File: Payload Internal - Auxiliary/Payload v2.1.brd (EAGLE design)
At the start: 90.5 x 91.8 mm, 11 parts, among them J30 M80-866XXXX, J31 M80-866XXXX

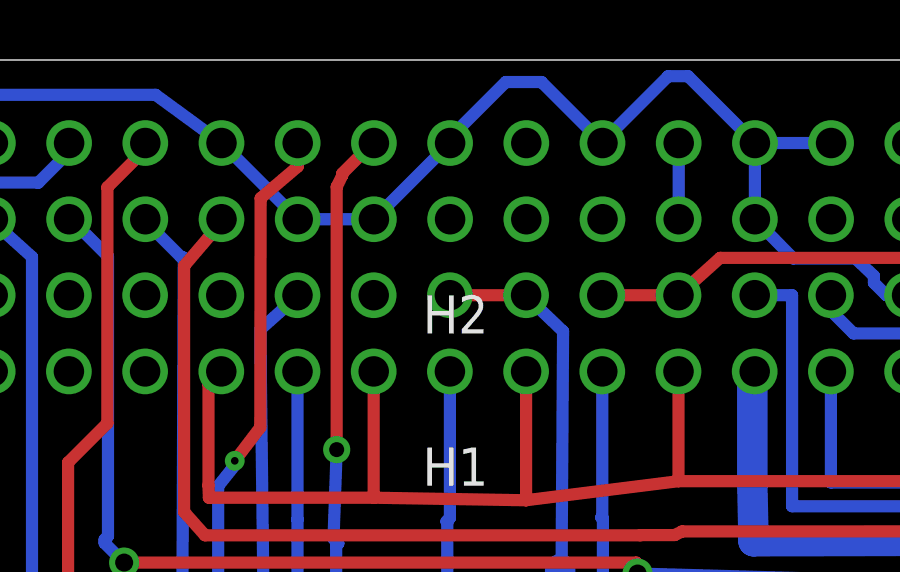
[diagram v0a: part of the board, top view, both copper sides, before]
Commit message: Revert "Fixed all the trivial wiring issues for the CDH, Diplexer, EPS and wiring harness schematics"
This reverts commits
  6713d85a6277b26f983fd7a52d0f95a7f9e4e046.
  086194ae58682b6763f31692a26cd4dac33df983
  82b42737f0fe6cd82dfea4a4ae7507beb01cc7b8

This revert is required because changing/connecting net names in eagle will automatically modify or destroy PCB traces associated with those netnames.
Updating the schematics and PCBs will need to be redone carefully to ensure no traces are destroyed.

	modified:   CDH-V3.7/CDH-v3.7.brd
	modified:   CDH-V3.7/CDH-v3.7.sch
	modified:   Diplexer/diplexer_v4rev0-schematic.sch
	modified:   EPS/eps-v1-0.brd
	modified:   EPS/eps-v1-0.sch
	modified:   Payload Internal - Auxiliary/Payload v2.1.brd
	modified:   Payload Internal - Auxiliary/Payload v2.1.sch
	modified:   Wiring Harness/wiring-harness-complete-v1.0.sch
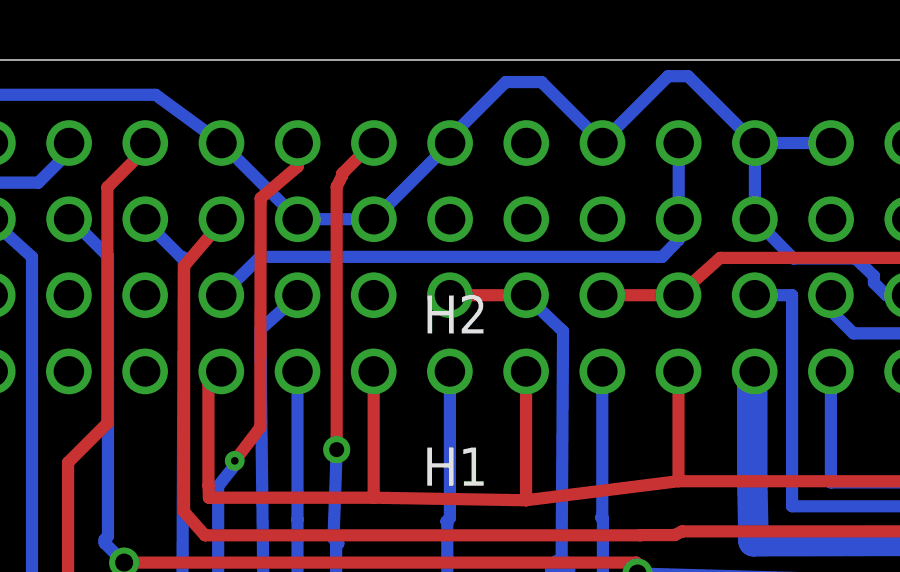
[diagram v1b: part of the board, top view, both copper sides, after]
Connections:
- net BATTERY_THRMSTOR1_+V renamed BATTERY_THRMSTOR_+V
- net BATTERY_THRMSTOR2_+V renamed BATTERY_THERMSTOR_2+
- net POW_9V renamed 9V
- net POW_RADIO_VBATT renamed POW_5V
- net THERMALGND1 renamed THERMALGND
- removed net EXTERNAL_POWER_V+: H2.52
- removed net N$1: H2.6
- removed net N$6: H2.10
- removed net POW_RADIO_3V3: H2.27, H2.28
- new net EXTERNAL_POWER_+V: H2.51
- new net N$19: H2.37
- new net N$89.: H2.21
- new net N$90: H2.23
- new net N$91: H2.25
- net EXTERNAL_POWER_GND: now also H2.52; no longer H2.51
- net N$4: now also H2.35; no longer H2.8
- net POW_RADIO_3.3V: now also H2.27, H2.28
- net Q6_SPI_SCLK: now also H2.6; no longer H2.21
- net Q6_SPI_SDI_MISO: now also H2.10; no longer H2.35
- net Q6_SPI_SDO_MOSI: now also H2.8; no longer H2.23
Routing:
- net POW_RADIO_3.3V: track 0.00 -> 19.2 mm
- net POW_RADIO_3V3: track 2.54 -> 0.00 mm
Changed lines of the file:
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@@
 <?xml version="1.0" encoding="utf-8"?>
 <!DOCTYPE eagle SYSTEM "eagle.dtd">
-<eagle version="7.3.0">
+<eagle version="7.2.0">
 <drawing>
 <settings>
@@
 <contactref element="H2" pad="47"/>
 </signal>
+<signal name="N$19">
+<contactref element="H2" pad="37"/>
+</signal>
 <signal name="N$22">
 <contactref element="H2" pad="34"/>
+</signal>
+<signal name="N$90">
+<contactref element="H2" pad="23"/>
 </signal>
 <signal name="N$27">
@@
 <contactref element="H1" pad="33"/>
 </signal>
+<signal name="Q6_SPI_SDO_MOSI">
+<contactref element="H2" pad="8"/>
+</signal>
 <signal name="Q6_SPI_CS1">
 <contactref element="H2" pad="12"/>
@@
 </polygon>
 </signal>
-<signal name="POW_RADIO_VBATT">
+<signal name="POW_5V">
 <contactref element="H1" pad="28"/>
 <contactref element="H1" pad="26"/>
@@
 <wire x1="81.331828125" y1="77.2444875" x2="82.066653125" y2="76.5096625" width="0.4064" layer="1"/>
 </signal>
+<signal name="N$89.">
+<contactref element="H2" pad="21"/>
+</signal>
+<signal name="Q6_SPI_SCLK">
+<contactref element="H2" pad="6"/>
+</signal>
+<signal name="Q6_SPI_SDI_MISO">
+<contactref element="H2" pad="10"/>
+</signal>
 <signal name="Q6_AIN_1">
 <contactref element="H1" pad="43"/>
@@
 <contactref element="H1" pad="51"/>
 </signal>
+<signal name="N$91">
+<contactref element="H2" pad="25"/>
+</signal>
 <signal name="POW_RADIO_3.3V">
+<contactref element="H2" pad="27"/>
 <contactref element="H1" pad="16"/>
+<contactref element="H2" pad="28"/>
+<wire x1="47.436940625" y1="89.05731875" x2="47.436940625" y2="86.51731875" width="0.4064" layer="16"/>
+<wire x1="47.436940625" y1="86.51731875" x2="47.436940625" y2="85.83329375" width="0.4064" layer="16"/>
+<wire x1="47.436940625" y1="85.83329375" x2="46.88775" y2="85.26289375" width="0.4064" layer="16"/>
+<wire x1="46.88775" y1="85.26289375" x2="33.48964375" y2="85.26289375" width="0.4064" layer="16"/>
+<wire x1="33.48964375" y1="85.26289375" x2="32.190153125" y2="83.9846125" width="0.4064" layer="16"/>
 </signal>
 <signal name="POW_3V3">
@@
 <contactref element="H1" pad="6"/>
 </signal>
-<signal name="BATTERY_THRMSTOR1_+V">
+<signal name="BATTERY_THRMSTOR_+V">
 <contactref element="H1" pad="8"/>
 </signal>
@@
 <contactref element="H2" pad="49"/>
 </signal>
-<signal name="Q6_SPI_SDI_MISO">
+<signal name="N$4">
 <contactref element="H2" pad="35"/>
 </signal>
-<signal name="EXTERNAL_POWER_V+">
+<signal name="EXTERNAL_POWER_GND">
 <contactref element="H2" pad="52"/>
 </signal>
@@
 <contactref element="H1" pad="13"/>
 </signal>
-<signal name="EXTERNAL_POWER_GND">
+<signal name="EXTERNAL_POWER_+V">
 <contactref element="H2" pad="51"/>
 </signal>
@@
 <contactref element="J31" pad="13"/>
 </signal>
-<signal name="THERMALGND1">
+<signal name="THERMALGND">
 <contactref element="H1" pad="5"/>
 <contactref element="J30" pad="9"/>
@@
 <contactref element="J31" pad="9"/>
 </signal>
-<signal name="N$60">
+<signal name="N$6">
 <via x="9.062225" y="88.85175625" extent="1-16" drill="3.3"/>
 </signal>
-<signal name="N$61">
+<signal name="N$7">
 <via x="82.728596875" y="88.855203125" extent="1-16" drill="3.3"/>
 </signal>
-<signal name="N$63">
+<signal name="N$8">
 <via x="85.261796875" y="3.130459375" extent="1-16" drill="3.3"/>
 </signal>
-<signal name="N$62">
+<signal name="N$9">
 <via x="5.259753125" y="3.12559375" extent="1-16" drill="3.3"/>
 </signal>
-<signal name="POW_9V">
+<signal name="9V">
 <contactref element="H1" pad="22"/>
 <contactref element="H1" pad="24"/>
@@
 <wire x1="45.01678125" y1="51.72485625" x2="45.1386375" y2="51.8467125" width="0.4064" layer="1"/>
 </signal>
-<signal name="N$654643543">
+<signal name="N$6546">
 <contactref element="H1" pad="14"/>
 </signal>
@@
 <wire x1="85.8217125" y1="50.10553125" x2="85.057015625" y2="50.10553125" width="0.4064" layer="1"/>
 </signal>
-<signal name="BATTERY_THRMSTOR2_+V">
+<signal name="BATTERY_THERMSTOR_2+">
 <contactref element="H1" pad="12"/>
 </signal>
-<signal name="POW_RADIO_3V3">
-<contactref element="H2" pad="27"/>
-<contactref element="H2" pad="28"/>
-<wire x1="47.436940625" y1="89.05731875" x2="47.436940625" y2="86.51731875" width="0.4064" layer="16"/>
-</signal>
-<signal name="N$6">
-<contactref element="H2" pad="10"/>
-</signal>
-<signal name="Q6_SPI_SDO_MOSI">
-<contactref element="H2" pad="23"/>
-</signal>
-<signal name="N$1">
-<contactref element="H2" pad="6"/>
-</signal>
-<signal name="N$4">
-<contactref element="H2" pad="8"/>
-</signal>
-<signal name="Q6_SPI_SCLK">
-<contactref element="H2" pad="21"/>
-</signal>
 </signals>

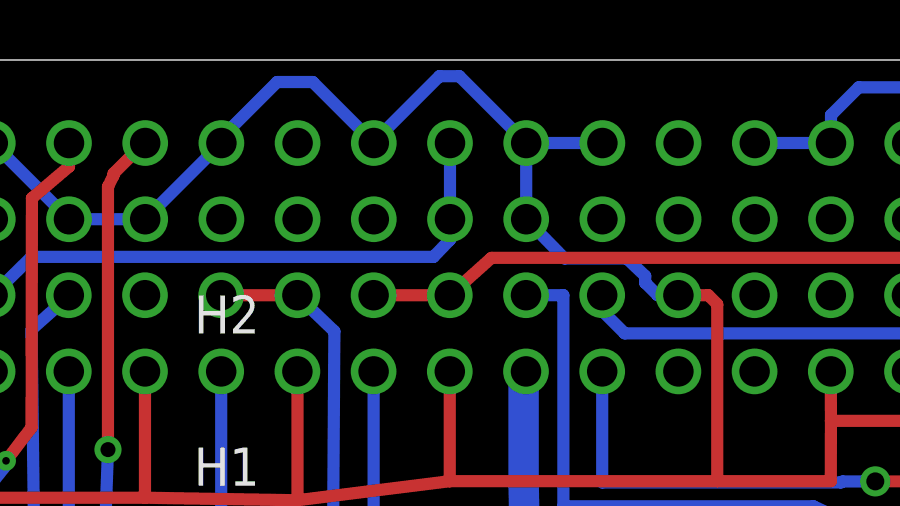
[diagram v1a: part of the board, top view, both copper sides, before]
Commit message: [CDH] updated trivial mismatches between connector netnames [EPS] updated trivial mismatches between connector netnames [PAYLOAD] updated trivial mismatches between connector netnames [WIRING] updated trivial mismatches between connector netnames
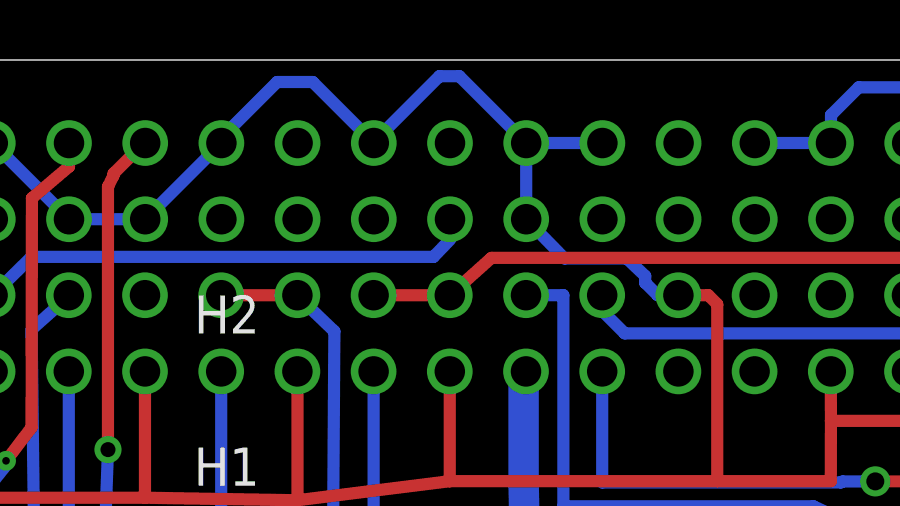
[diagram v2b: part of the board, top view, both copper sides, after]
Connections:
- net 9V renamed POW_9V
- net BATTERY_THERMSTOR_2+ renamed BATTERY_THRMSTOR2_+V
- net BATTERY_THRMSTOR_+V renamed BATTERY_THRMSTOR1_+V
- net POW_5V renamed POW_RADIO_VBATT
- net THERMALGND renamed THERMALGND1
- removed net EXTERNAL_POWER_+V: H2.51
- removed net N$19: H2.37
- removed net N$89.: H2.21
- removed net N$90: H2.23
- removed net N$91: H2.25
- new net EXTERNAL_POWER_V+: H2.52
- new net N$1: H2.6
- new net N$6: H2.10
- new net POW_RADIO_3V3: H2.27
- new net POW_RADIO_3V3_SYS: H2.28
- net EXTERNAL_POWER_GND: now also H2.51; no longer H2.52
- net N$4: now also H2.8; no longer H2.35
- net POW_RADIO_3.3V: no longer H2.27, H2.28
- net Q6_SPI_SCLK: now also H2.21; no longer H2.6
- net Q6_SPI_SDI_MISO: now also H2.35; no longer H2.10
- net Q6_SPI_SDO_MOSI: now also H2.23; no longer H2.8
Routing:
- net POW_RADIO_3.3V: track 19.2 -> 16.0 mm
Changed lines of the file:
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@@
 <?xml version="1.0" encoding="utf-8"?>
 <!DOCTYPE eagle SYSTEM "eagle.dtd">
-<eagle version="7.2.0">
+<eagle version="7.3.0">
 <drawing>
 <settings>
@@
 <contactref element="H2" pad="47"/>
 </signal>
-<signal name="N$19">
-<contactref element="H2" pad="37"/>
-</signal>
 <signal name="N$22">
 <contactref element="H2" pad="34"/>
-</signal>
-<signal name="N$90">
-<contactref element="H2" pad="23"/>
 </signal>
 <signal name="N$27">
@@
 <contactref element="H1" pad="33"/>
 </signal>
-<signal name="Q6_SPI_SDO_MOSI">
-<contactref element="H2" pad="8"/>
-</signal>
 <signal name="Q6_SPI_CS1">
 <contactref element="H2" pad="12"/>
@@
 </polygon>
 </signal>
-<signal name="POW_5V">
+<signal name="POW_RADIO_VBATT">
 <contactref element="H1" pad="28"/>
 <contactref element="H1" pad="26"/>
@@
 <wire x1="81.331828125" y1="77.2444875" x2="82.066653125" y2="76.5096625" width="0.4064" layer="1"/>
 </signal>
-<signal name="N$89.">
-<contactref element="H2" pad="21"/>
-</signal>
-<signal name="Q6_SPI_SCLK">
-<contactref element="H2" pad="6"/>
-</signal>
-<signal name="Q6_SPI_SDI_MISO">
-<contactref element="H2" pad="10"/>
-</signal>
 <signal name="Q6_AIN_1">
 <contactref element="H1" pad="43"/>
@@
 <contactref element="H1" pad="51"/>
 </signal>
-<signal name="N$91">
-<contactref element="H2" pad="25"/>
-</signal>
 <signal name="POW_RADIO_3.3V">
-<contactref element="H2" pad="27"/>
 <contactref element="H1" pad="16"/>
-<contactref element="H2" pad="28"/>
-<wire x1="47.436940625" y1="89.05731875" x2="47.436940625" y2="86.51731875" width="0.4064" layer="16"/>
-<wire x1="47.436940625" y1="86.51731875" x2="47.436940625" y2="85.83329375" width="0.4064" layer="16"/>
 <wire x1="47.436940625" y1="85.83329375" x2="46.88775" y2="85.26289375" width="0.4064" layer="16"/>
 <wire x1="46.88775" y1="85.26289375" x2="33.48964375" y2="85.26289375" width="0.4064" layer="16"/>
@@
 <contactref element="H1" pad="6"/>
 </signal>
-<signal name="BATTERY_THRMSTOR_+V">
+<signal name="BATTERY_THRMSTOR1_+V">
 <contactref element="H1" pad="8"/>
 </signal>
@@
 <contactref element="H2" pad="49"/>
 </signal>
-<signal name="N$4">
+<signal name="Q6_SPI_SDI_MISO">
 <contactref element="H2" pad="35"/>
 </signal>
-<signal name="EXTERNAL_POWER_GND">
+<signal name="EXTERNAL_POWER_V+">
 <contactref element="H2" pad="52"/>
 </signal>
@@
 <contactref element="H1" pad="13"/>
 </signal>
-<signal name="EXTERNAL_POWER_+V">
+<signal name="EXTERNAL_POWER_GND">
 <contactref element="H2" pad="51"/>
 </signal>
@@
 <contactref element="J31" pad="13"/>
 </signal>
-<signal name="THERMALGND">
+<signal name="THERMALGND1">
 <contactref element="H1" pad="5"/>
 <contactref element="J30" pad="9"/>
@@
 <contactref element="J31" pad="9"/>
 </signal>
-<signal name="N$6">
+<signal name="N$60">
 <via x="9.062225" y="88.85175625" extent="1-16" drill="3.3"/>
 </signal>
-<signal name="N$7">
+<signal name="N$61">
 <via x="82.728596875" y="88.855203125" extent="1-16" drill="3.3"/>
 </signal>
-<signal name="N$8">
+<signal name="N$63">
 <via x="85.261796875" y="3.130459375" extent="1-16" drill="3.3"/>
 </signal>
-<signal name="N$9">
+<signal name="N$62">
 <via x="5.259753125" y="3.12559375" extent="1-16" drill="3.3"/>
 </signal>
-<signal name="9V">
+<signal name="POW_9V">
 <contactref element="H1" pad="22"/>
 <contactref element="H1" pad="24"/>
@@
 <wire x1="45.01678125" y1="51.72485625" x2="45.1386375" y2="51.8467125" width="0.4064" layer="1"/>
 </signal>
-<signal name="N$6546">
+<signal name="N$654643543">
 <contactref element="H1" pad="14"/>
 </signal>
@@
 <wire x1="85.8217125" y1="50.10553125" x2="85.057015625" y2="50.10553125" width="0.4064" layer="1"/>
 </signal>
-<signal name="BATTERY_THERMSTOR_2+">
+<signal name="BATTERY_THRMSTOR2_+V">
 <contactref element="H1" pad="12"/>
 </signal>
+<signal name="POW_RADIO_3V3">
+<contactref element="H2" pad="27"/>
+</signal>
+<signal name="POW_RADIO_3V3_SYS">
+<contactref element="H2" pad="28"/>
+</signal>
+<signal name="N$6">
+<contactref element="H2" pad="10"/>
+</signal>
+<signal name="Q6_SPI_SDO_MOSI">
+<contactref element="H2" pad="23"/>
+</signal>
+<signal name="N$1">
+<contactref element="H2" pad="6"/>
+</signal>
+<signal name="N$4">
+<contactref element="H2" pad="8"/>
+</signal>
+<signal name="Q6_SPI_SCLK">
+<contactref element="H2" pad="21"/>
+</signal>
 </signals>

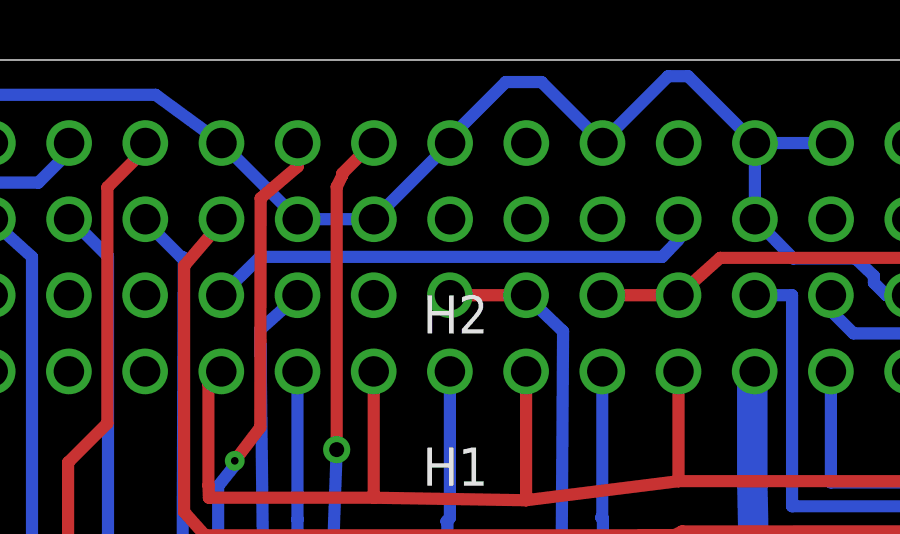
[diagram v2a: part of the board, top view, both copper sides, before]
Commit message: [PAYLOAD-INT] added h2 pin 26 and pin 28 short (to match actual PCB)
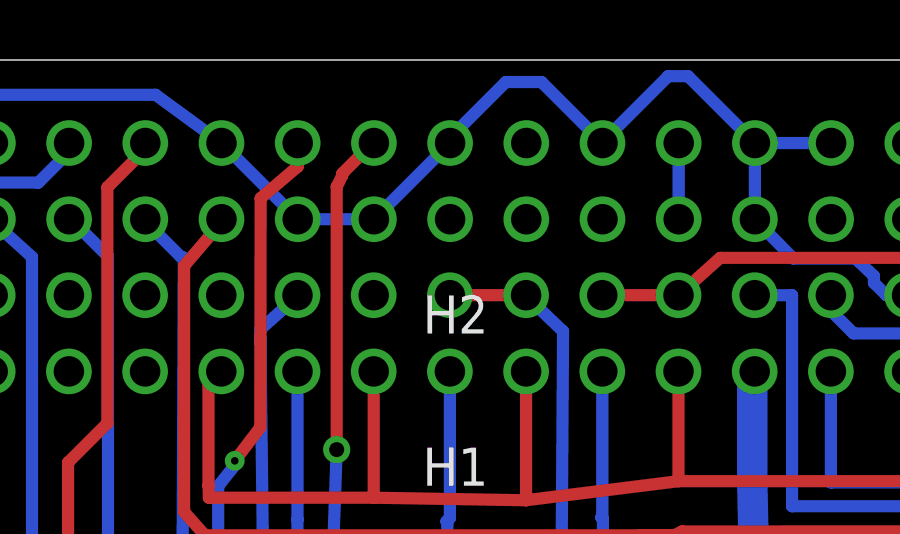
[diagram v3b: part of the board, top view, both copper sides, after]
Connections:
- removed net POW_RADIO_3V3_SYS: H2.28
- net POW_RADIO_3V3: now also H2.28
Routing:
- net POW_RADIO_3.3V: track 16.0 -> 0.00 mm
- net POW_RADIO_3V3: track 0.00 -> 2.54 mm
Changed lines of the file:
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@@
 <signal name="POW_RADIO_3.3V">
 <contactref element="H1" pad="16"/>
-<wire x1="47.436940625" y1="85.83329375" x2="46.88775" y2="85.26289375" width="0.4064" layer="16"/>
-<wire x1="46.88775" y1="85.26289375" x2="33.48964375" y2="85.26289375" width="0.4064" layer="16"/>
-<wire x1="33.48964375" y1="85.26289375" x2="32.190153125" y2="83.9846125" width="0.4064" layer="16"/>
 </signal>
 <signal name="POW_3V3">
@@
 <signal name="POW_RADIO_3V3">
 <contactref element="H2" pad="27"/>
-</signal>
-<signal name="POW_RADIO_3V3_SYS">
 <contactref element="H2" pad="28"/>
+<wire x1="47.436940625" y1="89.05731875" x2="47.436940625" y2="86.51731875" width="0.4064" layer="16"/>
 </signal>
 <signal name="N$6">
